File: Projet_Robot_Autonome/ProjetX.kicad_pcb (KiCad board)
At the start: 4 copper layers, 57 x 54 mm, 99 parts, among them IC1 MP1475DJ-LF-P, J1 Conn_ST_STDC14, J11 Conn_01x05, J2 Screw_Terminal_01x02, J3 Conn_01x06, J4 BORDER, J5 Conn_01x06, J6 Conn_01x05, J7 BORDER, J8 BORDER, J9 BORDER, SW1 ON/OFF, SW2 SW_Push, U1 STM32G431CBUx, U2 ZXBM5210-SP, U3 ZXBM5210-SP, U4 ADXL343, Y1 Crystal_GND24_Small

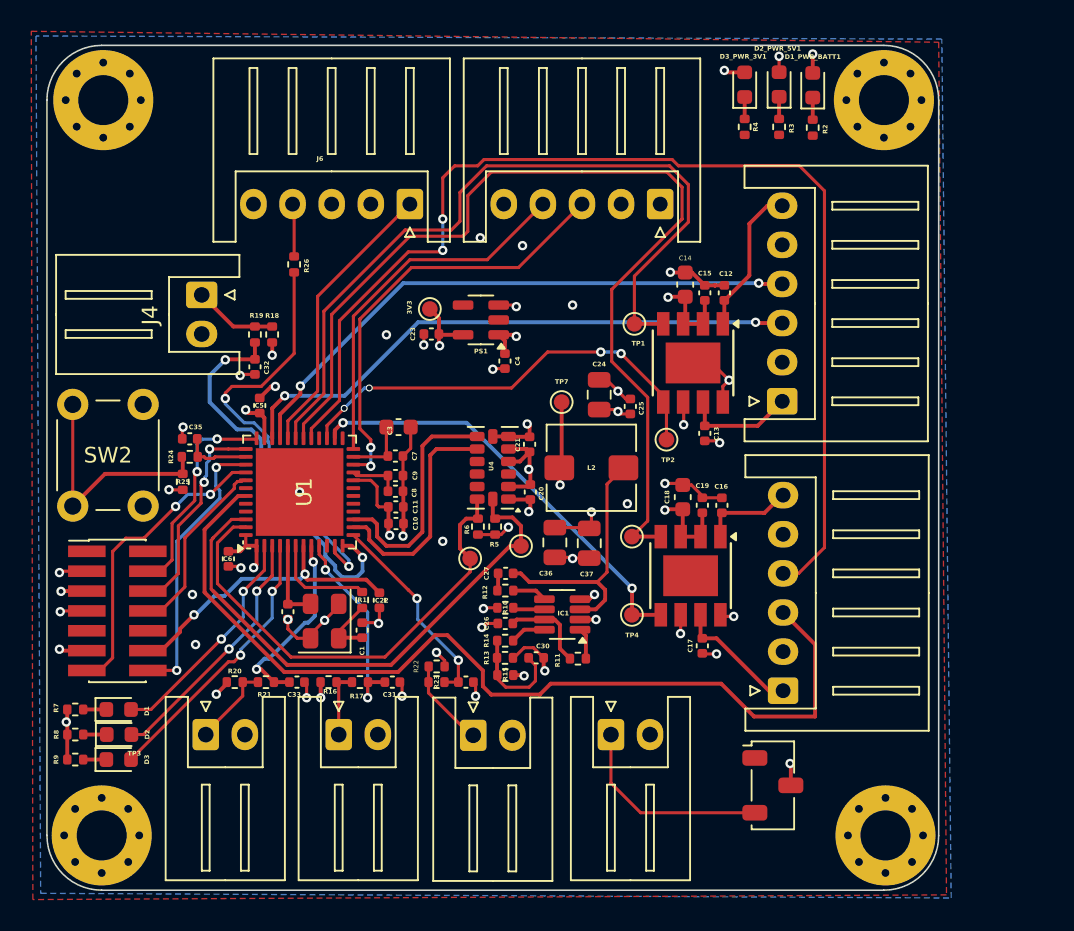
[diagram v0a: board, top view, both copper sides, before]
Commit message: Updated KiCad project files
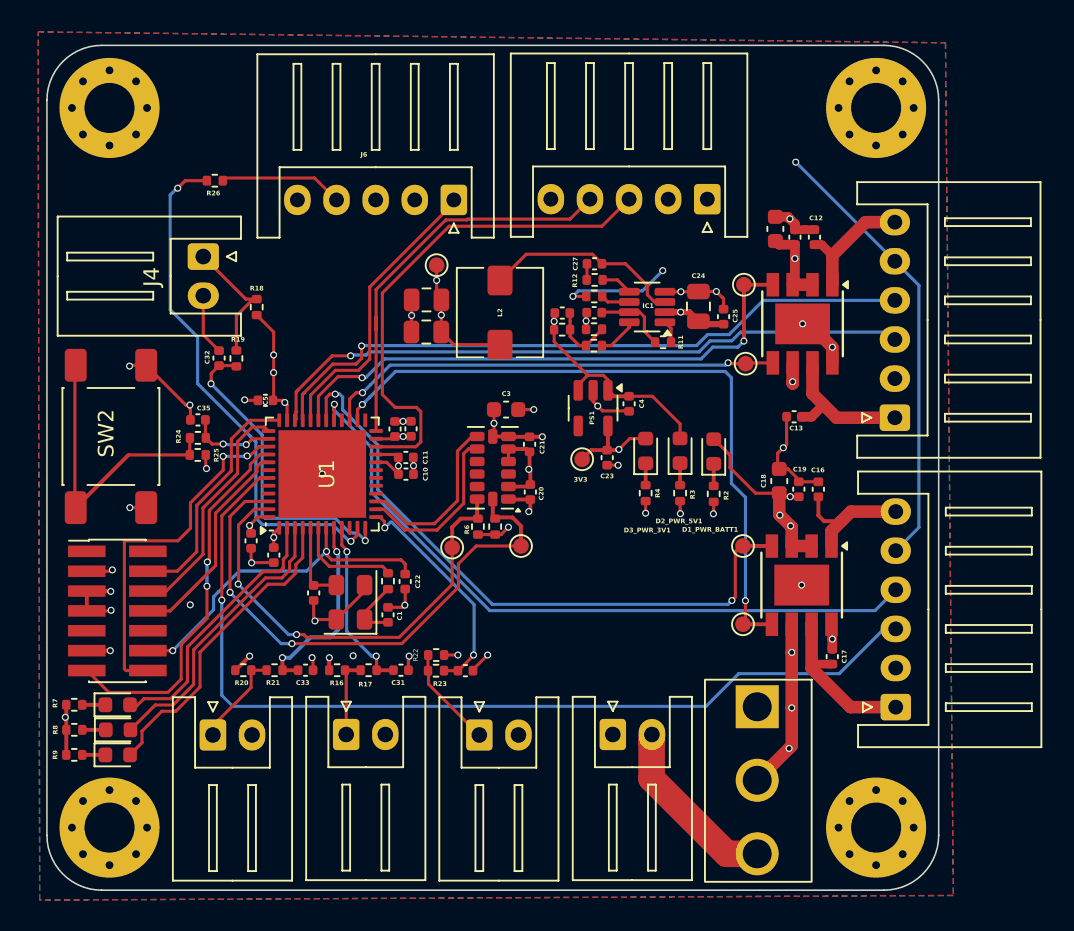
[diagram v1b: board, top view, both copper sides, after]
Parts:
- removed SW1: ON/OFF, Button_Switch_SMD:Nidec_Copal_CAS-120A
- added S1: 1101M2S3CQE2, swithes:sw wurth, F.Cu at (179.8, 121.6)
- SW2: footprint Button_Switch_THT:SW_PUSH_6mm_H9.5mm -> Button_Switch_SMD:SW_Push_1P1T_NO_E-Switch_TL3301NxxxxxG
- moved H3 49.6 mm to (139.0, 125.0)
- moved H4 49.5 mm to (188.0, 125.0)
- moved R3 24.3 mm to (175.5, 103.6)
- moved D2_PWR_5V1 24.3 mm to (175.5, 100.9)
- moved D1_PWR_BATT1 24.3 mm to (177.6, 101.0)
- moved D3_PWR_3V1 24.3 mm to (173.3, 100.9)
- moved R2 24.3 mm to (177.6, 103.7)
- moved R4 24.3 mm to (173.3, 103.6)
- moved R15 22.8 mm to (170.0, 93.1), turned to 0 degrees
- moved C30 22.1 mm to (167.9, 92.1), turned to 180 degrees
- moved R13 21.3 mm to (167.9, 93.2), turned to 180 degrees
- moved R11 20.9 mm to (174.4, 94.0)
- moved R10 20.7 mm to (170.0, 91.0)
- moved R12 20.7 mm to (170.0, 90.0)
- moved C26 20.7 mm to (170.0, 92.1)
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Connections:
- J2 pad 1: Net-(J2-Pin_1) -> GND
- J2 pad 2: GND -> Net-(J2-Pin_2)
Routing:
- net /Actionneurs/ENCOD_B2: track 73.2 -> 44.9 mm, vias 2 -> 1
- net +3.3V: track 39.8 -> 67.7 mm, vias 14 -> 18
- net /Actionneurs/FWD2: track 64.0 -> 41.0 mm, vias 0 -> 2
- net +BATT: track 21.0 -> 42.1 mm, vias 9 -> 11
- net /Actionneurs/REV2: track 27.6 -> 43.8 mm
- net /Actionneurs/FWD1: track 49.8 -> 35.8 mm, vias 0 -> 2
- net Net-(J2-Pin_1): track 13.1 -> 0.00 mm
- net Net-(J2-Pin_2): track 0.00 -> 11.6 mm
- net GND: track 62.4 -> 72.7 mm, vias 38 -> 36
- net +5V: track 15.8 -> 23.6 mm, vias 6 -> 3
- net /STM32/LIDAR_TX: track 27.1 -> 33.4 mm
- net /STM32/BLE_RX: track 28.1 -> 33.5 mm, vias 2 -> 0
- net /Actionneurs/ENCOD_A1: track 36.8 -> 42.0 mm, vias 2 -> 1
- net /Actionneurs/ENCOD_B1: track 37.4 -> 42.4 mm, vias 2 -> 1
- net /STM32/BORDER_4: track 25.3 -> 20.4 mm
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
